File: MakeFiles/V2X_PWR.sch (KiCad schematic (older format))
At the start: 68 parts, among them P10 Ficudial3, P11 Ficudial4, P12 Ficudial1, P13 Ficudial2, P14 Ficudial3, P15 Ficudial4, P3 USB_A, P4 Board Mount 1, P5 Board Mount 2, P6 Board Mount 3, P7 Board Mount 4, P8 Ficudial1, P9 Ficudial2, Q11 IRF9335, Q12 IRF9335, SW2 SW_PUSH, U10 FDC6326L, U11 TLV70012DCK, U12 TLV70012DCK, U13 TLV70012DCK, U7 FDC6326L, U8 XRP6124, U9 XRP6124

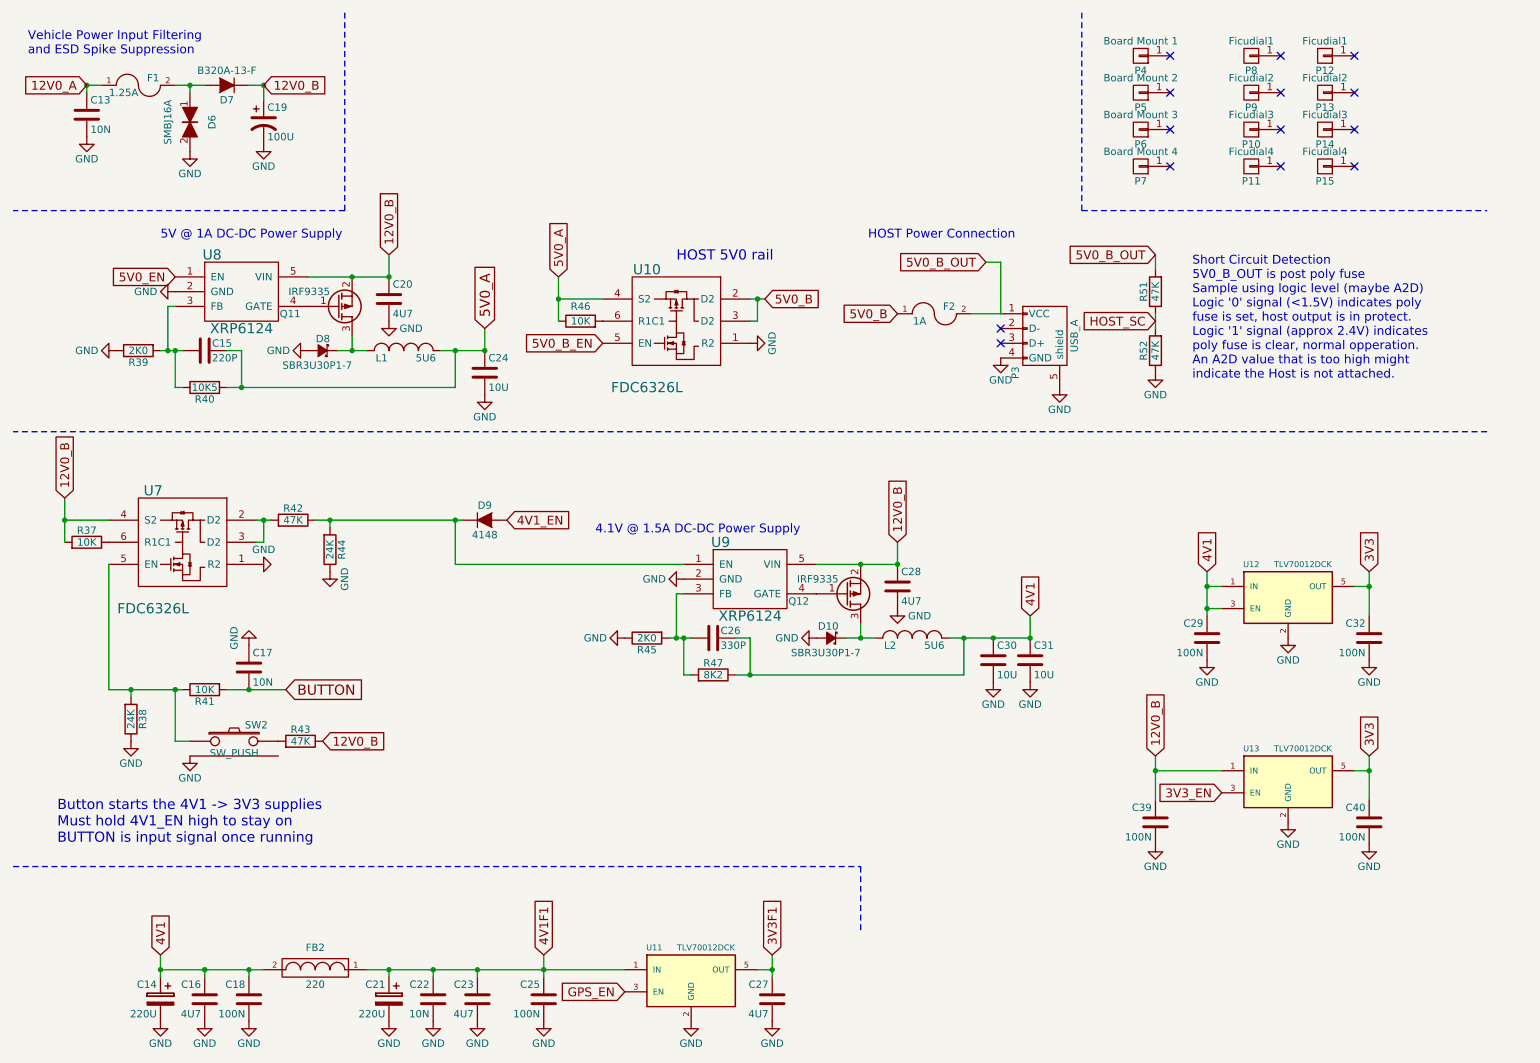
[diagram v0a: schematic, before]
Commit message: Changes for documentation
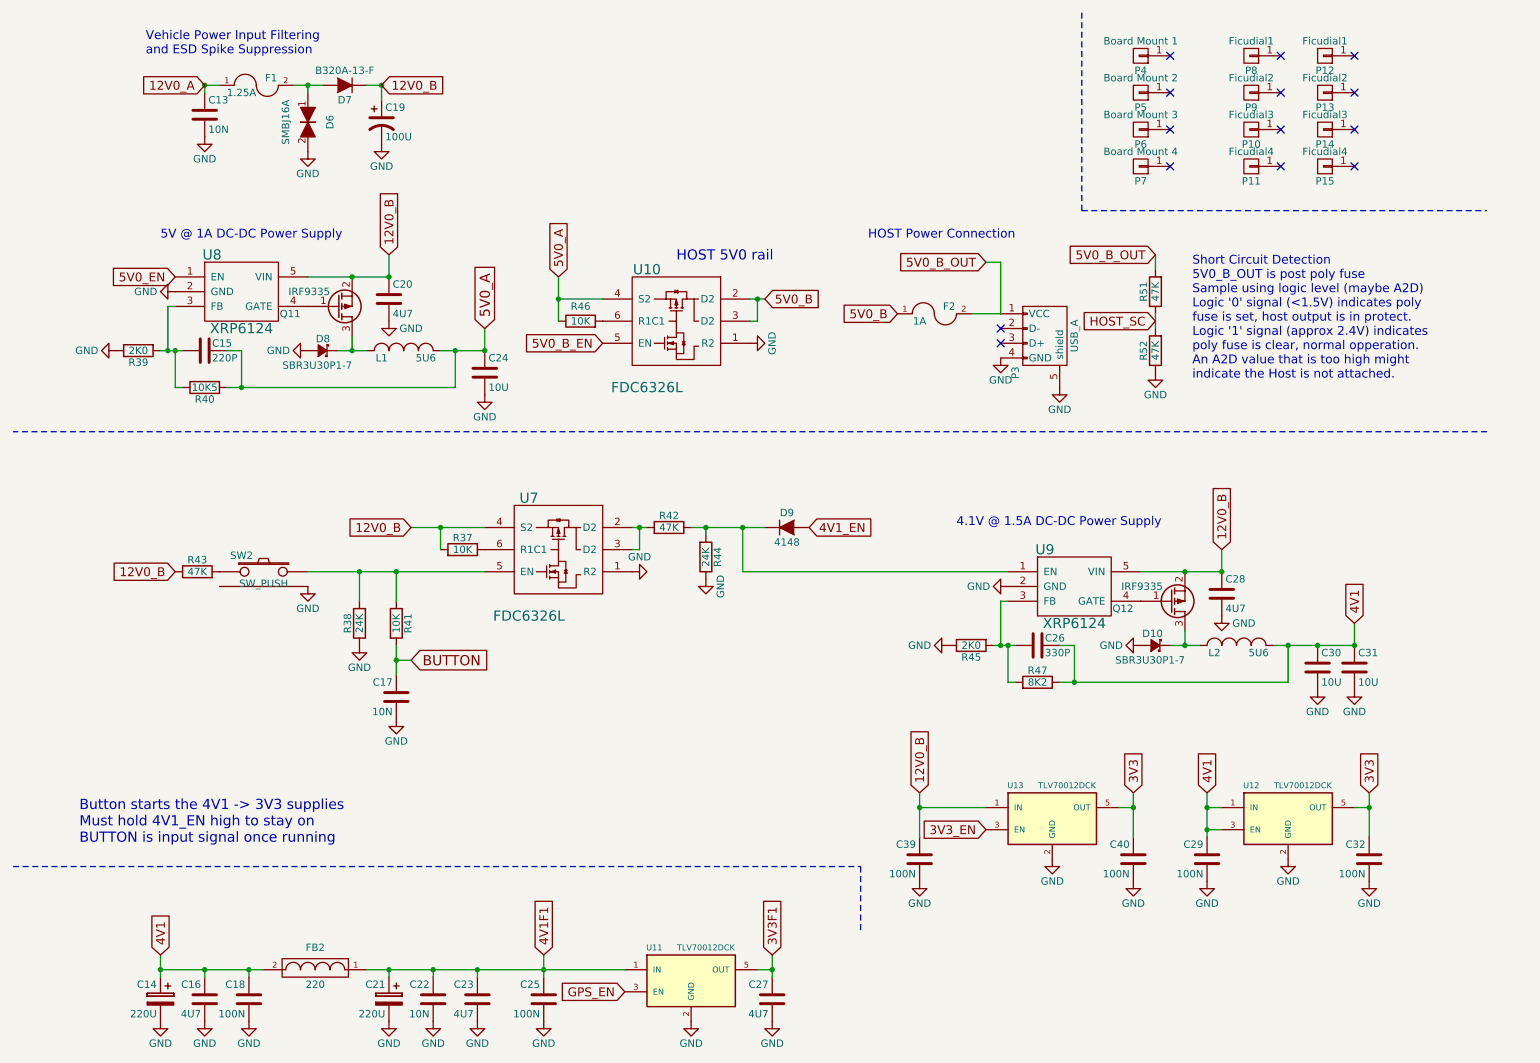
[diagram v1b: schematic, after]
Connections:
- net BUTTON: now also C17.1; no longer C17.2
- net GND: now also C17.2; no longer C17.1
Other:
- moved on the sheet: C13, C17, C19, C26, C28, C29, C30, C31, C32, C39, C40, D10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
